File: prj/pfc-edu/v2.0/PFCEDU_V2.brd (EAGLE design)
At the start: 403.9 x 355.1 mm, 238 parts, among them IC2 PCA9615DP, IC3 PCA9615DP, J2 54602-908LF, J3 54602-908LF, Q1 MMBT2222A, Q2 MMBT2222A, Q3 MMBT2222A, Q4 MMBT2222A, Q5 MMBT2222A, T1 R-78E5.0-1.0, T2 R-78E12.0-1.0, U1 TCA9548APWRPW24-M, U10 HPP845E034R5, U11 SHT25, U12 T6713-5K, U17 LM2937IMP3.3NOPB, U2 STD12NF06LT4, U20 RCD-24-0.70/VREF, U21 RCD-24-0.70/VREF, U22 RCD-24-0.70/VREF, U23 RCD-24-0.70/VREF, U24 RCD-24-0.70/VREF, U25 RCD-24-0.70/VREF, U27 DAC5578SPW, U3 STD12NF06LT4, U30 PCA9685, U4 PCF8574APWRPW20-M, U5 STD12NF06LT4, U6 STD12NF06LT4, U7 STD12NF06LT4, U9 CCS811

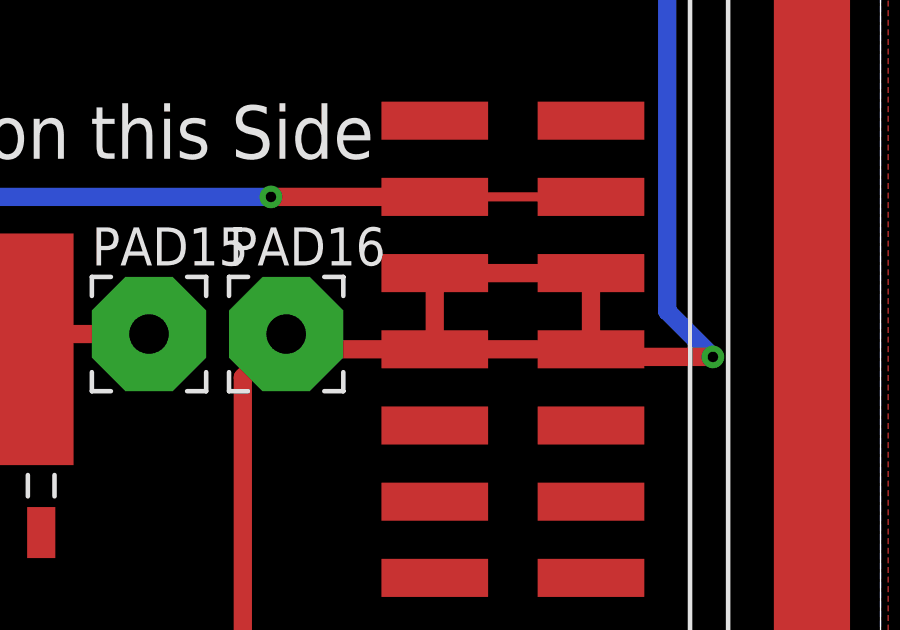
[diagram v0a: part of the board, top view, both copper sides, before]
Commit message: PCB update
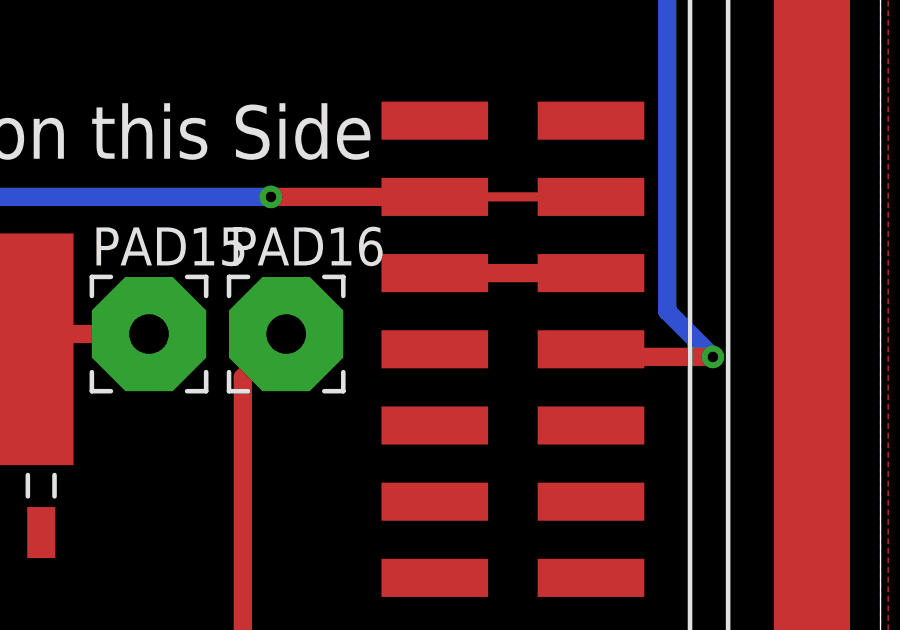
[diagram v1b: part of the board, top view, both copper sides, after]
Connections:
- net +5V: no longer U$4.SYS5V, U$4.SYS5V1
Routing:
- net +5V: track 419.1 -> 404.0 mm
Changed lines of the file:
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@@
 <?xml version="1.0" encoding="utf-8"?>
 <!DOCTYPE eagle SYSTEM "eagle.dtd">
-<eagle version="9.0.1">
+<eagle version="9.1.1">
 <drawing>
 <settings>
@@
 <param name="checkStop" value="0"/>
 <param name="checkValues" value="0"/>
+<param name="checkNames" value="1"/>
+<param name="checkWireStubs" value="1"/>
+<param name="checkPolygonWidth" value="0"/>
 <param name="useDiameter" value="13"/>
 <param name="maxErrors" value="50"/>
@@
 <contactref element="U$4" pad="VDD5V1"/>
 <contactref element="U$4" pad="VDD5V"/>
-<contactref element="U$4" pad="SYS5V"/>
-<contactref element="U$4" pad="SYS5V1"/>
 <wire x1="171.6938375" y1="262.93318125" x2="268.43481875" y2="262.93318125" width="0.6096" layer="16"/>
 <wire x1="268.43481875" y1="262.93318125" x2="277.622" y2="253.746" width="0.6096" layer="16"/>
@@
 <via x="279.146" y="225.044" extent="1-16" drill="0.35"/>
 <wire x1="279.146" y1="225.044" x2="275.336" y2="225.044" width="0.6096" layer="1"/>
-<wire x1="275.336" y1="225.044" x2="275.082" y2="225.298" width="0.6096" layer="1"/>
-<wire x1="275.082" y1="225.298" x2="275.082" y2="227.838" width="0.6096" layer="1"/>
 <wire x1="275.082" y1="227.838" x2="269.875" y2="227.838" width="0.6096" layer="1"/>
-<wire x1="269.875" y1="227.838" x2="269.875" y2="225.298" width="0.6096" layer="1"/>
-<wire x1="269.875" y1="225.298" x2="275.082" y2="225.298" width="0.6096" layer="1"/>
 <contactref element="PAD16" pad="1"/>
-<wire x1="269.875" y1="225.298" x2="265.43" y2="225.298" width="0.6096" layer="1"/>
 <wire x1="265.43" y1="225.298" x2="264.922" y2="225.806" width="0.6096" layer="1"/>
 <contactref element="PAD18" pad="1"/>
@@
 <wire x1="263.477" y1="209.41588125" x2="263.477" y2="224.361" width="0.6096" layer="1"/>
 <wire x1="263.477" y1="224.361" x2="264.922" y2="225.806" width="0.6096" layer="1"/>
+<wire x1="275.336" y1="225.044" x2="275.082" y2="227.838" width="0" layer="19" extent="1-1"/>
+<wire x1="44.792" y1="250.444" x2="47.498" y2="249.936" width="0" layer="19" extent="1-1"/>
+<wire x1="43.448" y1="247.2944" x2="44.792" y2="250.444" width="0" layer="19" extent="1-1"/>
+<wire x1="47.244" y1="246.38" x2="47.498" y2="249.936" width="0" layer="19" extent="1-1"/>
+<wire x1="46.228" y1="243.84" x2="46.99" y2="246.126" width="0" layer="19" extent="1-1"/>
+<wire x1="47.752" y1="242.316" x2="46.228" y2="243.84" width="0" layer="19" extent="1-1"/>
+<wire x1="45.974" y1="240.538" x2="47.752" y2="242.316" width="0" layer="19" extent="1-1"/>
+<wire x1="265.43" y1="225.298" x2="269.875" y2="227.838" width="0" layer="19" extent="1-1"/>
 </signal>
 <signal name="N$12">
@@
 </signal>
 </signals>
+<mfgpreviewcolors>
+<mfgpreviewcolor name="soldermaskcolor" color="0xC8008000"/>
+<mfgpreviewcolor name="silkscreencolor" color="0xFFFEFEFE"/>
+<mfgpreviewcolor name="backgroundcolor" color="0xFF282828"/>
+<mfgpreviewcolor name="coppercolor" color="0xFFFFBF00"/>
+<mfgpreviewcolor name="substratecolor" color="0xFF786E46"/>
+</mfgpreviewcolors>
 <errors>
 </errors>
